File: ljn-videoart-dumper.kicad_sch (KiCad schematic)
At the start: 8 parts, among them J1 Power, J2 Digital/PWM, J3 Analog, J4 Digital/PWM, J5 Video Art Edge, U1 74HC165, U2 74HC595, U3 74HC595

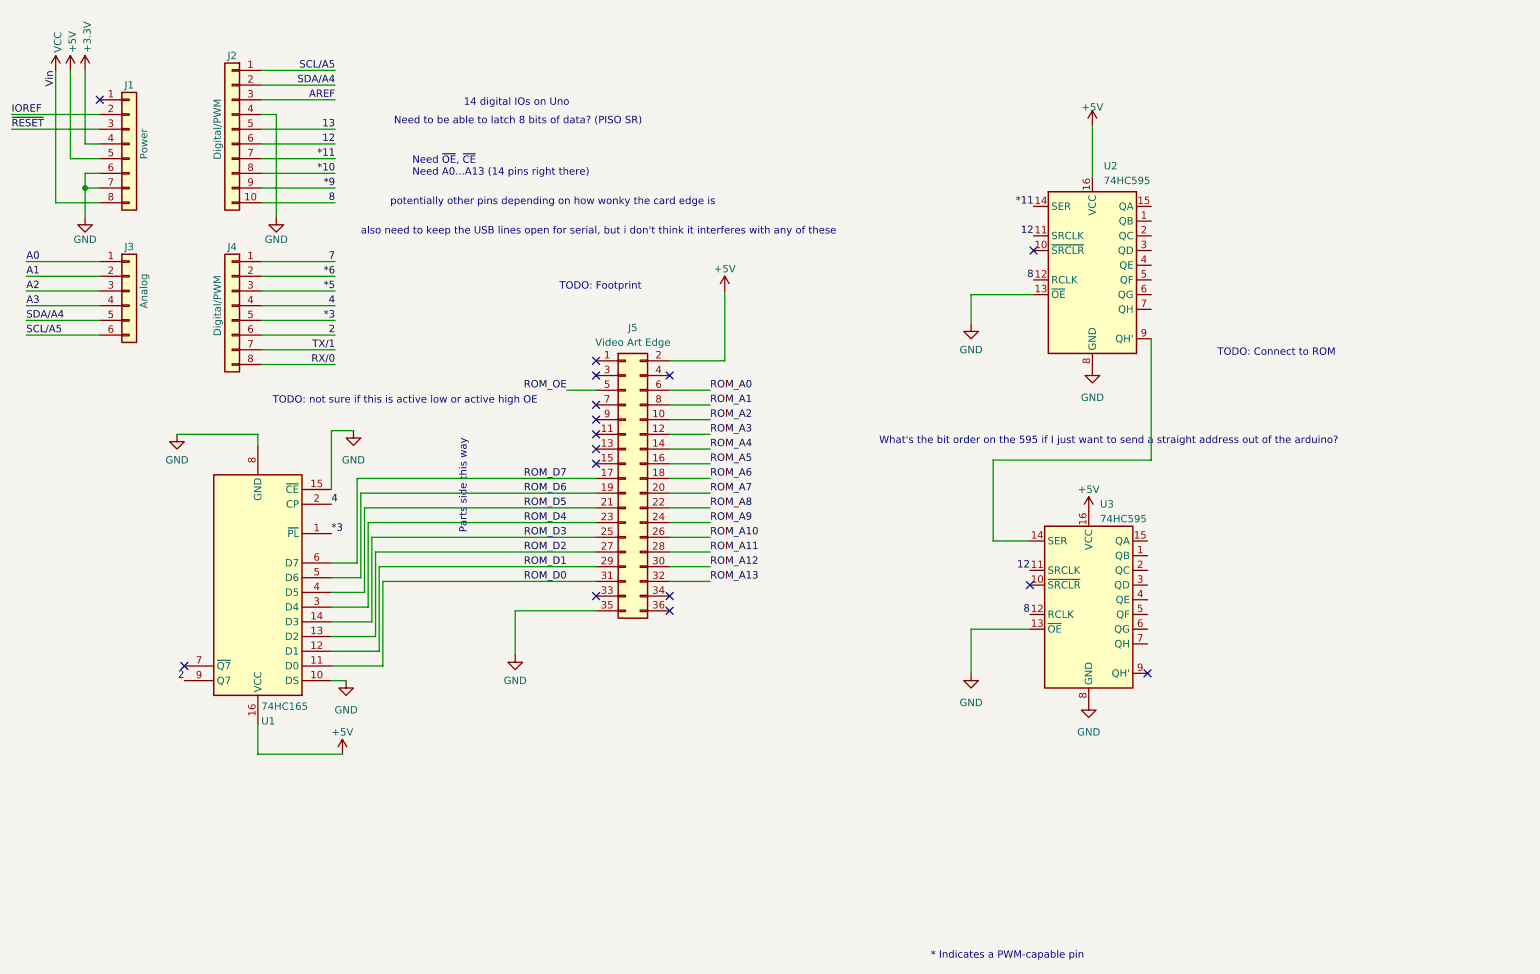
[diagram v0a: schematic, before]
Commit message: Final re-route
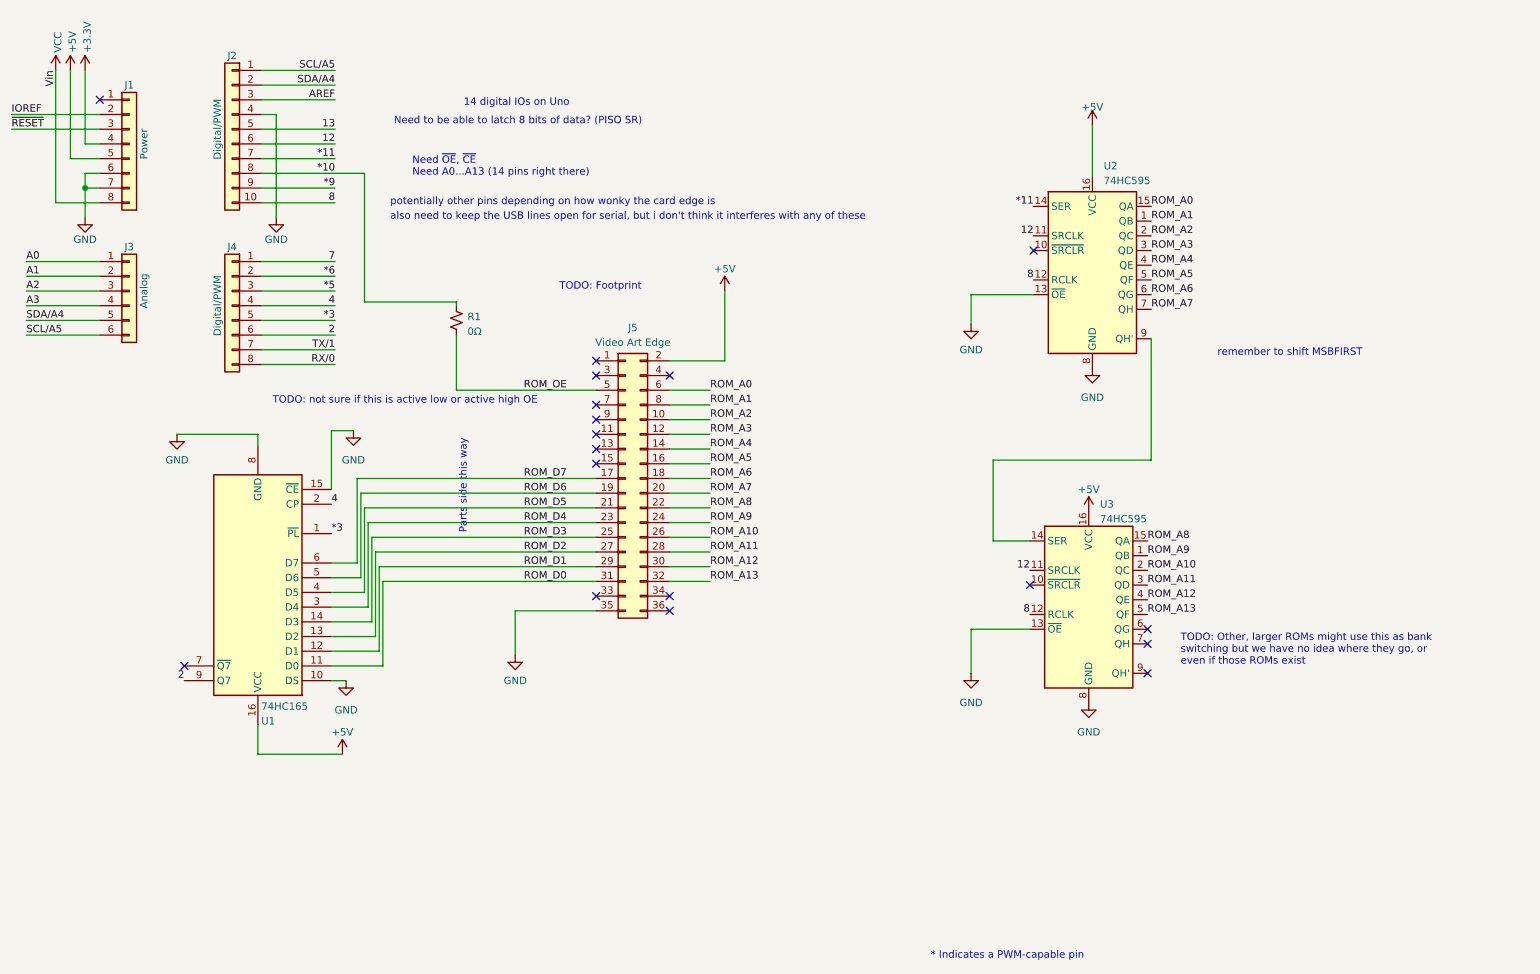
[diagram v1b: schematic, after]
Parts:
- added R1: 0Ω, Resistor_THT:R_Axial_DIN0207_L6.3mm_D2.5mm_P10.16mm_Horizontal, symbol Device:R_Small_US
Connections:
- net *10: now also R1.1
- net ROM_A0: now also U2.15 (QA)
- net ROM_A1: now also U2.1 (QB)
- net ROM_A10: now also U3.2 (QC)
- net ROM_A11: now also U3.3 (QD)
- net ROM_A12: now also U3.4 (QE)
- net ROM_A13: now also U3.5 (QF)
- net ROM_A2: now also U2.2 (QC)
- net ROM_A3: now also U2.3 (QD)
- net ROM_A4: now also U2.4 (QE)
- net ROM_A5: now also U2.5 (QF)
- net ROM_A6: now also U2.6 (QG)
- net ROM_A7: now also U2.7 (QH)
- net ROM_A8: now also U3.15 (QA)
- net ROM_A9: now also U3.1 (QB)
- net ROM_OE: now also R1.2
- no-connect marks 16 -> 18
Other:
- note added: "TODO: Other, larger ROMs might use this as bank switching but we have no idea where they go, or even if those ROMs exist"
- note added: "remember to shift MSBFIRST"
- note removed: "TODO: Connect to ROM"
- note removed: "What's the bit order on the 595 if I just want to send a straight address out of the arduino?"
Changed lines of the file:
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@@
   (no_connect (at 132.715 120.015))
   (no_connect (at 48.895 129.54))
+  (no_connect (at 215.265 125.73))
   (no_connect (at 120.015 79.375))
   (no_connect (at 132.715 79.375))
@@
   (no_connect (at 120.015 76.835))
   (no_connect (at 120.015 86.995))
+  (no_connect (at 215.265 123.19))
   (no_connect (at 194.945 115.57))
   (no_connect (at 34.29 31.75))
@@
     (stroke (width 0) (type solid))
   )
-  (wire (pts (xy 62.23 44.45) (xy 74.93 44.45))
+  (wire (pts (xy 62.23 44.45) (xy 80.01 44.45))
     (stroke (width 0) (type solid))
   )
@@
     (stroke (width 0) (type solid))
   )
+  (wire (pts (xy 80.01 66.675) (xy 80.01 44.45))
+    (stroke (width 0) (type default))
+  )
   (wire (pts (xy 74.295 129.54) (xy 83.185 129.54))
     (stroke (width 0) (type default))
@@
     (stroke (width 0) (type default))
   )
+  (wire (pts (xy 95.885 66.675) (xy 80.01 66.675))
+    (stroke (width 0) (type default))
+  )
   (wire (pts (xy 132.715 84.455) (xy 139.7 84.455))
     (stroke (width 0) (type default))
@@
     (stroke (width 0) (type default))
   )
+  (wire (pts (xy 95.885 72.39) (xy 95.885 81.915))
+    (stroke (width 0) (type default))
+  )
   (wire (pts (xy 34.29 64.77) (xy 21.59 64.77))
     (stroke (width 0) (type solid))
@@
     (stroke (width 0) (type solid))
   )
-  (wire (pts (xy 114.935 81.915) (xy 120.015 81.915))
+  (wire (pts (xy 95.885 81.915) (xy 120.015 81.915))
     (stroke (width 0) (type default))
   )
@@
     (stroke (width 0) (type default))
   )
+  (wire (pts (xy 95.885 66.675) (xy 95.885 67.31))
+    (stroke (width 0) (type default))
+  )
   (wire (pts (xy 80.645 104.775) (xy 120.015 104.775))
     (stroke (width 0) (type default))
@@
     (stroke (width 0) (type solid))
   )
-  (text "TODO: Connect to ROM" (at 227.33 76.2 0)
-    (effects (font (size 1.27 1.27)) (justify left bottom))
-  )
-  (text "What's the bit order on the 595 if I just want to send a straight address out of the arduino?"
-    (at 168.91 91.44 0)
+  (text "remember to shift MSBFIRST" (at 227.33 76.2 0)
     (effects (font (size 1.27 1.27)) (justify left bottom))
   )
@@
   )
   (text "also need to keep the USB lines open for serial, but i don't think it interferes with any of these"
-    (at 79.375 55.245 0)
+    (at 84.455 52.705 0)
+    (effects (font (size 1.27 1.27)) (justify left bottom))
+  )
+  (text "TODO: Other, larger ROMs might use this as bank\nswitching but we have no idea where they go, or\neven if those ROMs exist"
+    (at 220.98 129.54 0)
     (effects (font (size 1.27 1.27)) (justify left bottom))
   )
@@
     (effects (font (size 1.27 1.27)) (justify right bottom))
   )
+  (label "ROM_A0" (at 215.9 50.165 0) (fields_autoplaced)
+    (effects (font (size 1.27 1.27)) (justify left bottom))
+  )
   (label "2" (at 74.93 72.39 180) (fields_autoplaced)
     (effects (font (size 1.27 1.27)) (justify right bottom))
@@
     (effects (font (size 1.27 1.27)) (justify left bottom))
   )
+  (label "ROM_A3" (at 215.9 57.785 0) (fields_autoplaced)
+    (effects (font (size 1.27 1.27)) (justify left bottom))
+  )
+  (label "ROM_A11" (at 215.265 115.57 0) (fields_autoplaced)
+    (effects (font (size 1.27 1.27)) (justify left bottom))
+  )
   (label "13" (at 74.93 36.83 180) (fields_autoplaced)
     (effects (font (size 1.27 1.27)) (justify right bottom))
   )
+  (label "ROM_A6" (at 215.9 65.405 0) (fields_autoplaced)
+    (effects (font (size 1.27 1.27)) (justify left bottom))
+  )
+  (label "ROM_A7" (at 215.9 67.945 0) (fields_autoplaced)
+    (effects (font (size 1.27 1.27)) (justify left bottom))
+  )
   (label "ROM_A11" (at 139.7 109.855 0) (fields_autoplaced)
     (effects (font (size 1.27 1.27)) (justify left bottom))
@@
     (effects (font (size 1.27 1.27)) (justify left bottom))
   )
+  (label "ROM_A1" (at 215.9 52.705 0) (fields_autoplaced)
+    (effects (font (size 1.27 1.27)) (justify left bottom))
+  )
   (label "ROM_A13" (at 139.7 114.935 0) (fields_autoplaced)
     (effects (font (size 1.27 1.27)) (justify left bottom))
@@
     (effects (font (size 1.27 1.27)) (justify right bottom))
   )
+  (label "ROM_A13" (at 215.265 120.65 0) (fields_autoplaced)
+    (effects (font (size 1.27 1.27)) (justify left bottom))
+  )
   (label "ROM_OE" (at 114.935 81.915 180) (fields_autoplaced)
     (effects (font (size 1.27 1.27)) (justify right bottom))
@@
     (effects (font (size 1.27 1.27)) (justify right bottom))
   )
+  (label "ROM_A9" (at 215.265 110.49 0) (fields_autoplaced)
+    (effects (font (size 1.27 1.27)) (justify left bottom))
+  )
   (label "ROM_A1" (at 139.7 84.455 0) (fields_autoplaced)
     (effects (font (size 1.27 1.27)) (justify left bottom))
@@
     (effects (font (size 1.27 1.27)) (justify right bottom))
   )
+  (label "ROM_A10" (at 215.265 113.03 0) (fields_autoplaced)
+    (effects (font (size 1.27 1.27)) (justify left bottom))
+  )
   (label "A1" (at 21.59 62.23 0) (fields_autoplaced)
     (effects (font (size 1.27 1.27)) (justify left bottom))
@@
     (effects (font (size 1.27 1.27)) (justify left bottom))
   )
+  (label "ROM_A12" (at 215.265 118.11 0) (fields_autoplaced)
+    (effects (font (size 1.27 1.27)) (justify left bottom))
+  )
   (label "A0" (at 21.59 59.69 0) (fields_autoplaced)
     (effects (font (size 1.27 1.27)) (justify left bottom))
@@
     (effects (font (size 1.27 1.27)) (justify right bottom))
   )
+  (label "ROM_A8" (at 215.265 107.95 0) (fields_autoplaced)
+    (effects (font (size 1.27 1.27)) (justify left bottom))
+  )
   (label "*11" (at 195.58 50.165 180) (fields_autoplaced)
     (effects (font (size 1.27 1.27)) (justify right bottom))
   )
+  (label "ROM_A4" (at 215.9 60.325 0) (fields_autoplaced)
+    (effects (font (size 1.27 1.27)) (justify left bottom))
+  )
   (label "Vin" (at 26.67 26.67 270) (fields_autoplaced)
     (effects (font (size 1.27 1.27)) (justify right bottom))
@@
     (effects (font (size 1.27 1.27)) (justify left bottom))
   )
+  (label "ROM_A2" (at 215.9 55.245 0) (fields_autoplaced)
+    (effects (font (size 1.27 1.27)) (justify left bottom))
+  )
   (label "ROM_A0" (at 139.7 81.915 0) (fields_autoplaced)
     (effects (font (size 1.27 1.27)) (justify left bottom))
@@
   (label "ROM_D4" (at 114.935 104.775 180) (fields_autoplaced)
     (effects (font (size 1.27 1.27)) (justify right bottom))
+  )
+  (label "ROM_A5" (at 215.9 62.865 0) (fields_autoplaced)
+    (effects (font (size 1.27 1.27)) (justify left bottom))
   )
   (symbol (lib_id "Connector_Generic:Conn_01x08") (at 39.37 39.37 0) (unit 1)
@@
         )
       )
+    )
+  )
+  (symbol (lib_id "Device:R_Small_US") (at 95.885 69.85 0) (unit 1)
+    (in_bom yes) (on_board yes) (dnp no) (fields_autoplaced)
+    (property "Reference" "R1" (at 97.79 69.215 0)
+      (effects (font (size 1.27 1.27)) (justify left))
+    )
+    (property "Value" "0Ω" (at 97.79 71.755 0)
+      (effects (font (size 1.27 1.27)) (justify left))
+    )
+    (property "Footprint" "Resistor_THT:R_Axial_DIN0207_L6.3mm_D2.5mm_P10.16mm_Horizontal" (at 95.885 69.85 0)
+      (effects (font (size 1.27 1.27)) hide)
+    )
+    (property "Datasheet" "~" (at 95.885 69.85 0)
+      (effects (font (size 1.27 1.27)) hide)
+    )
+    (pin "1")
+    (pin "2")
+    (instances
+      (project "ljn-videoart-dumper"
+        (path "/e63e39d7-6ac0-4ffd-8aa3-1841a4541b55"
+          (reference "R1") (unit 1)
+        )
+      )
